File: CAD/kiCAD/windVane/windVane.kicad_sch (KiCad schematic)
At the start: 10 parts

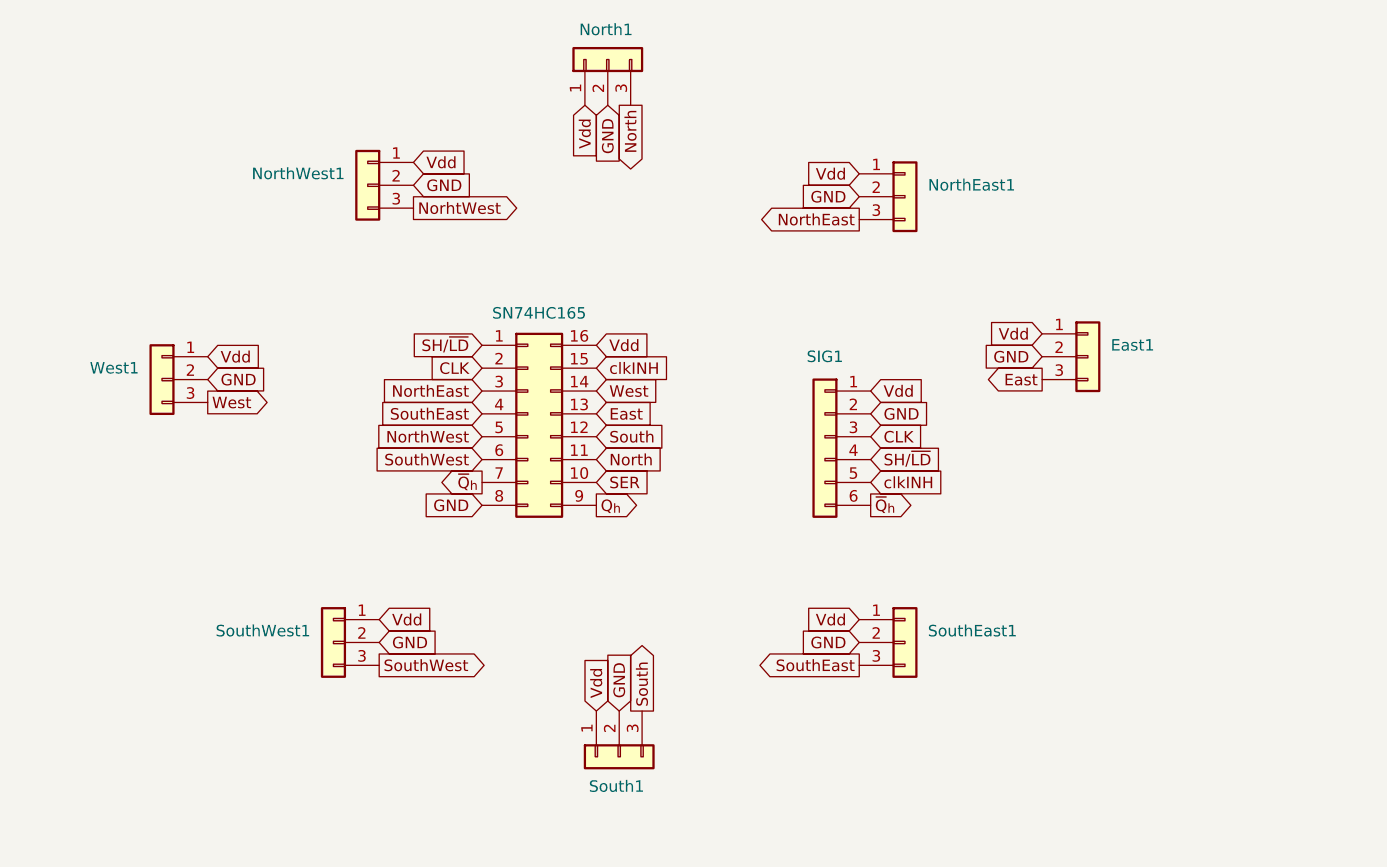
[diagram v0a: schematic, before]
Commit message: Update Schematics
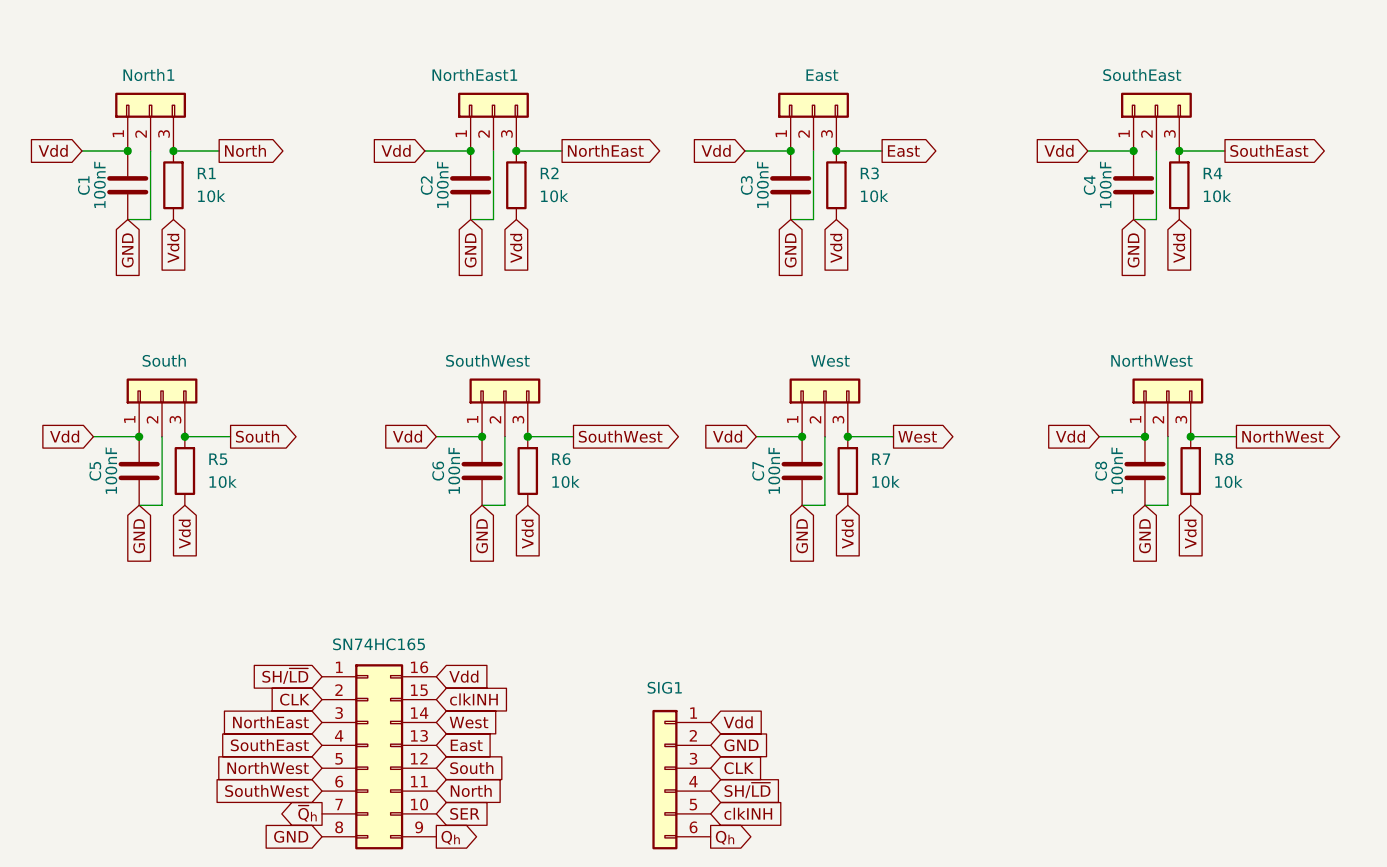
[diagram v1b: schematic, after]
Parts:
- removed East1, NorthWest1, South1, SouthEast1, SouthWest1, West1: Conn_01x03, Connector_PinHeader_2.54mm:PinHeader_1x03_P2.54mm_Vertical, symbol Connector_Generic:Conn_01x03
- added C1, C2, C3, C4, C5, C6, C7, C8: 100nF, symbol Device:C
- added East, NorthWest, South, SouthEast, SouthWest, West: Conn_01x03, Connector_PinHeader_2.54mm:PinHeader_1x03_P2.54mm_Vertical, symbol Connector_Generic:Conn_01x03
- added R1, R2, R3, R4, R5, R6, R7, R8: 10k, symbol Device:R
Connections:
- net East: now also East.3 (Pin_3), R3.2
- net GND: now also C1.1, C2.1, C3.1, C4.1, C5.1, C6.1, C7.1, C8.1, East.2 (Pin_2), NorthWest.2 (Pin_2), South.2 (Pin_2), SouthEast.2 (Pin_2), SouthWest.2 (Pin_2), West.2 (Pin_2)
- net North: now also R1.2
- net NorthEast: now also R2.2
- net NorthWest: now also NorthWest.3 (Pin_3), R8.2
- net Q_{h}: now also SIG1.6 (Pin_6)
- net South: now also R5.2, South.3 (Pin_3)
- net SouthEast: now also R4.2, SouthEast.3 (Pin_3)
- net SouthWest: now also R6.2, SouthWest.3 (Pin_3)
- net Vdd: now also C1.2, C2.2, C3.2, C4.2, C5.2, C6.2, C7.2, C8.2, East.1 (Pin_1), NorthWest.1 (Pin_1), R1.1, R2.1, R3.1, R4.1, R5.1, R6.1, R7.1, R8.1, South.1 (Pin_1), SouthEast.1 (Pin_1), SouthWest.1 (Pin_1), West.1 (Pin_1)
- net West: now also R7.2, West.3 (Pin_3)
- net ~{Q}_{h}: no longer SIG1.6 (Pin_6)
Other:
- moved on the sheet: North1, SIG1, SN74HC165
